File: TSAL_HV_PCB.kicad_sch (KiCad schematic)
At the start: 41 parts, among them J3 Conn_01x03_Socket, J4 Conn_01x03_Socket, K1 SPU01M-5, Q2 2N7002, Q3 2N7002, U1 LM393, U2 4N35, U3 TPS7B88-Q1

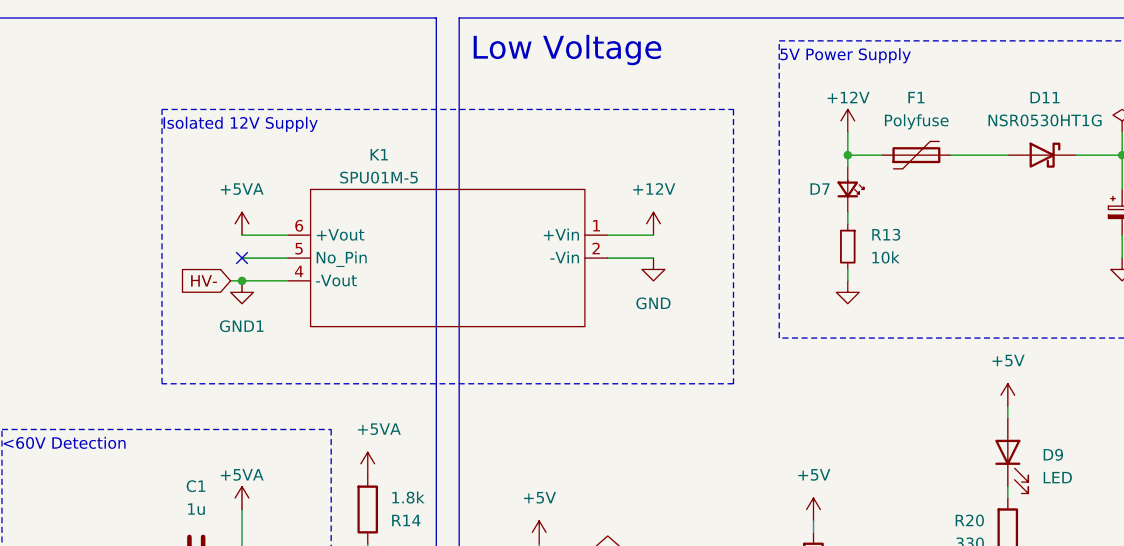
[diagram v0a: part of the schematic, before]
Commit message: Polyfuse for DC-DC supply
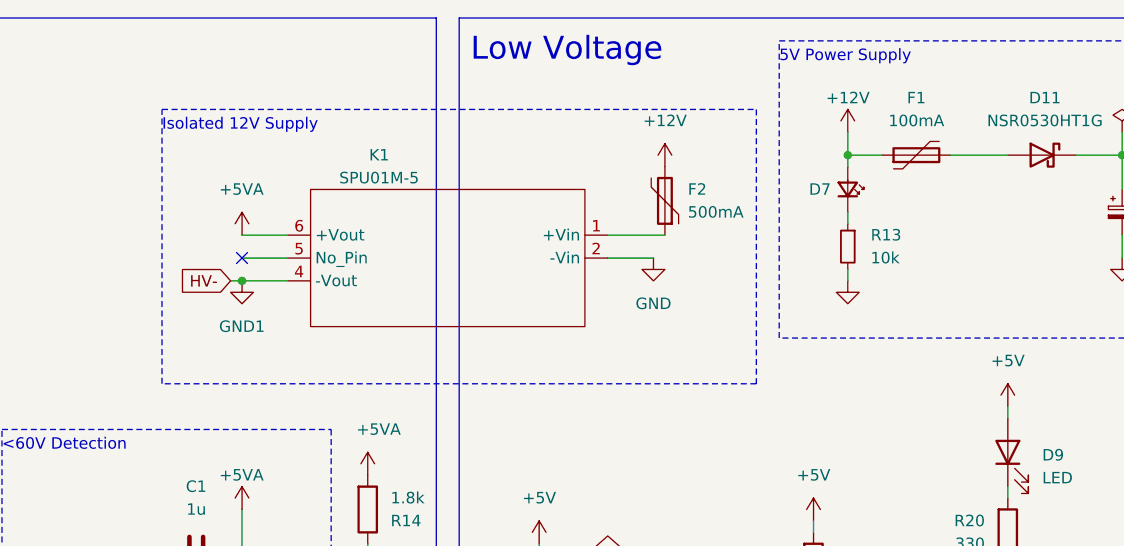
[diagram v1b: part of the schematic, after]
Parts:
- added F2: 500mA, Resistor_SMD:R_0805_2012Metric, symbol Device:Polyfuse
- F1: value Polyfuse -> 100mA
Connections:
- net +12V: now also F2.2; no longer K1.1 (+Vin)
- new net: F2.1, K1.1 (+Vin)
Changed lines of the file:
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@@
 	(rectangle
 		(start 116.84 27.94)
-		(end 180.34 58.42)
+		(end 182.88 58.42)
 		(stroke
 			(width 0)
@@
 	(wire
 		(pts
-			(xy 166.37 41.91) (xy 171.45 41.91)
+			(xy 201.93 85.09) (xy 203.2 85.09)
 		)
 		(stroke
@@
 	(wire
 		(pts
-			(xy 201.93 85.09) (xy 203.2 85.09)
+			(xy 241.3 72.39) (xy 242.57 72.39)
 		)
 		(stroke
@@
 	(wire
 		(pts
-			(xy 241.3 72.39) (xy 242.57 72.39)
+			(xy 193.04 30.48) (xy 193.04 33.02)
 		)
 		(stroke
@@
 	(wire
 		(pts
-			(xy 193.04 30.48) (xy 193.04 33.02)
+			(xy 172.72 41.91) (xy 166.37 41.91)
 		)
 		(stroke
@@
 	(symbol
 		(lib_id "power:+12V")
-		(at 171.45 41.91 0)
+		(at 172.72 34.29 0)
 		(unit 1)
 		(exclude_from_sim no)
@@
 		(fields_autoplaced yes)
 		(property "Reference" "#PWR019"
-			(at 171.45 45.72 0)
+			(at 172.72 38.1 0)
 			(effects
 				(font
@@
 		)
 		(property "Value" "+12V"
-			(at 171.45 36.83 0)
+			(at 172.72 29.21 0)
 			(effects
 				(font
@@
 		)
 		(property "Footprint" ""
-			(at 171.45 41.91 0)
+			(at 172.72 34.29 0)
 			(effects
 				(font
@@
 		)
 		(property "Datasheet" ""
-			(at 171.45 41.91 0)
+			(at 172.72 34.29 0)
 			(effects
 				(font
@@
 		)
 		(property "Description" ""
-			(at 171.45 41.91 0)
+			(at 172.72 34.29 0)
 			(effects
 				(font
@@
 			)
 		)
-		(property "Value" "Polyfuse"
+		(property "Value" "100mA"
 			(at 200.66 29.21 90)
 			(effects
@@
 					(unit 1)
 				)
+			)
+		)
+	)
+	(symbol
+		(lib_id "Device:Polyfuse")
+		(at 172.72 38.1 180)
+		(unit 1)
+		(exclude_from_sim no)
+		(in_bom yes)
+		(on_board yes)
+		(dnp no)
+		(fields_autoplaced yes)
+		(property "Reference" "F2"
+			(at 175.26 36.8299 0)
+			(effects
+				(font
+					(size 1.27 1.27)
+				)
+				(justify right)
+			)
+		)
+		(property "Value" "500mA"
+			(at 175.26 39.3699 0)
+			(effects
+				(font
+					(size 1.27 1.27)
+				)
+				(justify right)
+			)
+		)
+		(property "Footprint" "Resistor_SMD:R_0805_2012Metric"
+			(at 171.45 33.02 0)
+			(effects
+				(font
+					(size 1.27 1.27)
+				)
+				(justify left)
+				(hide yes)
+			)
+		)
+		(property "Datasheet" "~"
+			(at 172.72 38.1 0)
+			(effects
+				(font
+					(size 1.27 1.27)
+				)
+				(hide yes)
+			)
+		)
+		(property "Description" "Resettable fuse, polymeric positive temperature coefficient"
+			(at 172.72 38.1 0)
+			(effects
+				(font
+					(size 1.27 1.27)
+				)
+				(hide yes)
+			)
+		)
+		(pin "2"
+		)
+		(pin "1"
+		)
+		(instances
+			(project "TSAL_HV_PCB"
+				(path "/49aa962b-9fa6-407b-842a-3cf8300a05dc"
+					(reference "F2")
+					(unit 1)
+				)
